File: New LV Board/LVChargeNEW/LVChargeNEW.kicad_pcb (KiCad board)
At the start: 2 copper layers, 54 parts, among them Q1 CSD15380F3T, Q2 CSD15380F3T, Q3 CSD15380F3T, Q4 CSD15380F3T, U1 PQ25856QWRRVRQ1

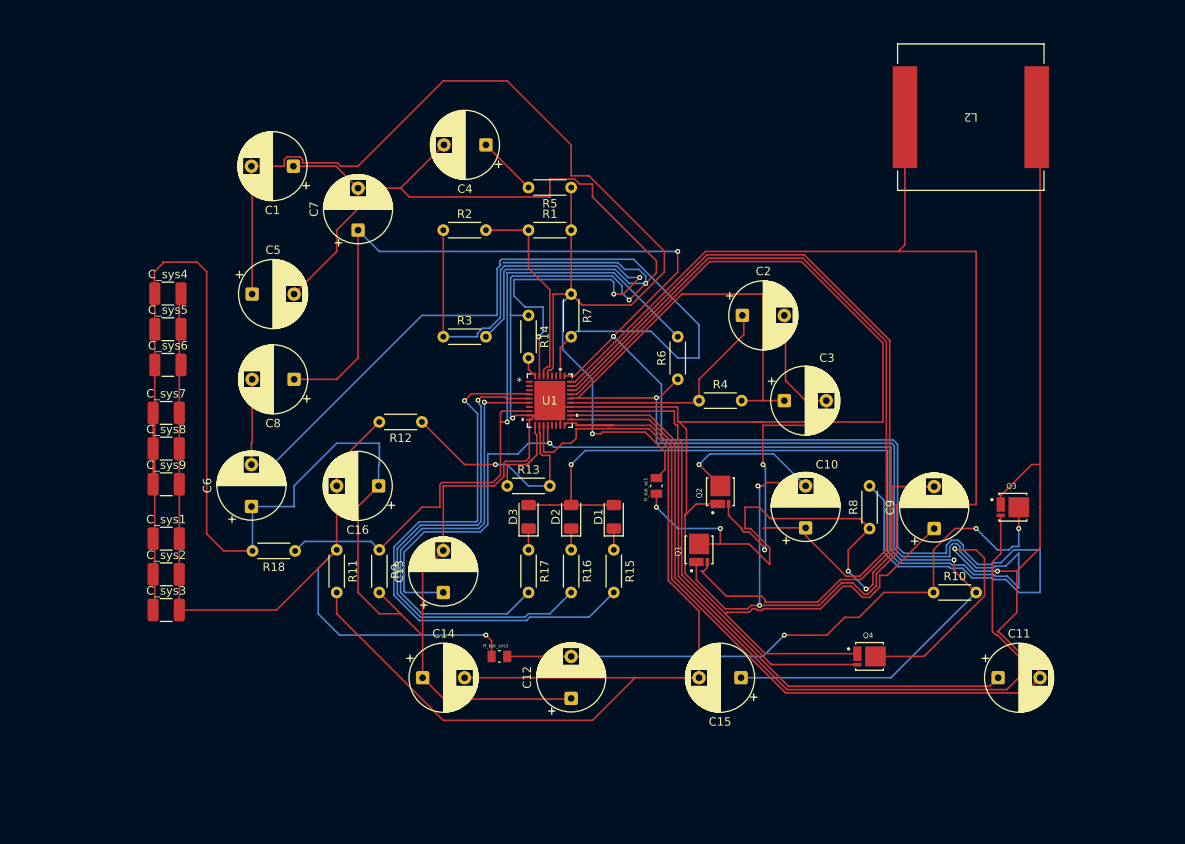
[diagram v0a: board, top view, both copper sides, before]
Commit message: updated LVCharge
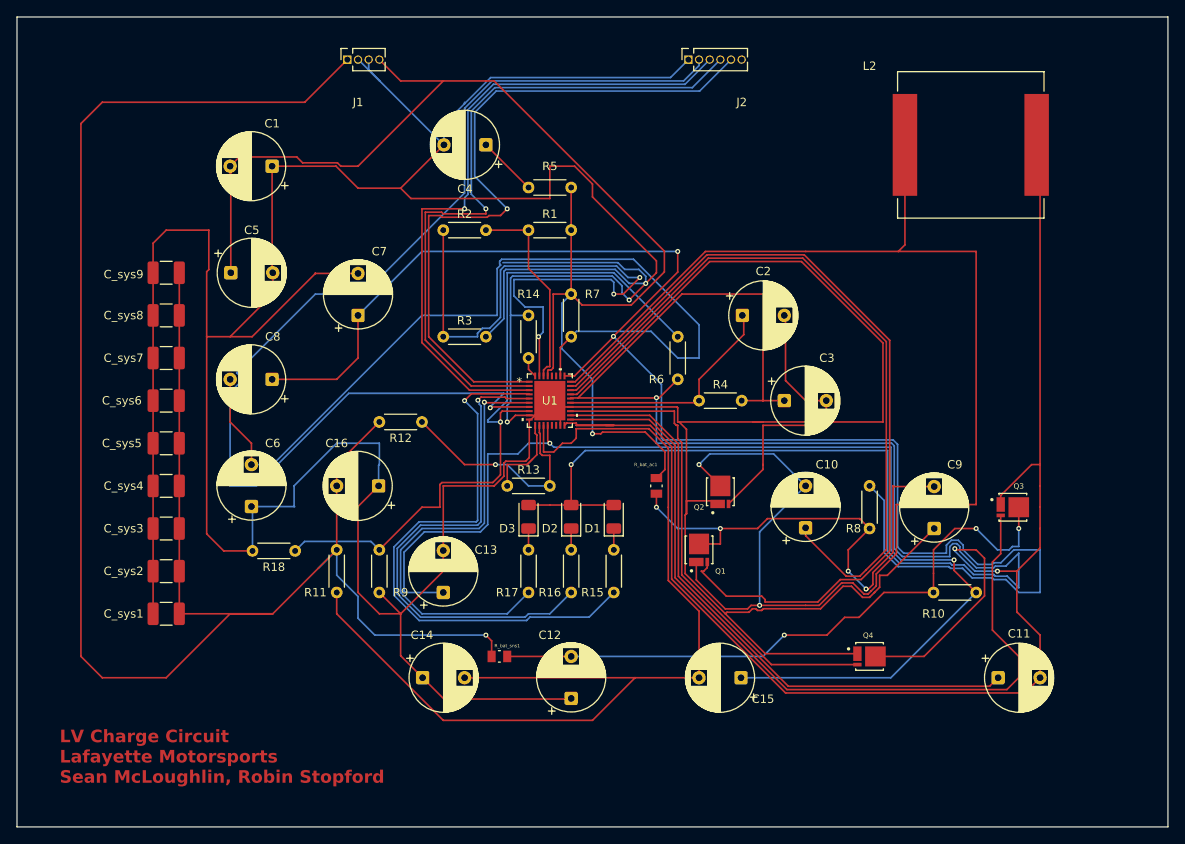
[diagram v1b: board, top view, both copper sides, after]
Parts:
- added J1: Conn_01x04_Socket, Connector_PinSocket_1.27mm:PinSocket_1x04_P1.27mm_Vertical, F.Cu at (80.0, 50.8)
- added J2: Conn_01x05_Socket, Connector_PinSocket_1.27mm:PinSocket_1x06_P1.27mm_Vertical, F.Cu at (120.7, 50.8)
- moved C_sys9 25.2 mm to (58.4, 76.2)
- moved C_sys4 22.9 mm to (58.4, 101.6)
- moved C_sys8 15.9 mm to (58.4, 81.3)
- moved C_sys5 13.6 mm to (58.4, 96.5)
- moved C7 10.2 mm to (81.3, 81.3)
- moved C_sys3 9.71 mm to (58.4, 106.7)
- moved C_sys1 8.95 mm to (58.4, 116.8)
- moved C_sys7 6.55 mm to (58.4, 86.4)
- moved C_sys6 4.26 mm to (58.4, 91.4)
- moved C5 3.59 mm to (66.1, 76.2)
- moved L2 3.30 mm to (154.3, 61.0)
- moved C8 2.62 mm to (71.0, 88.9)
- moved C1 2.54 mm to (71.0, 63.5)
- moved C_sys2 0.38 mm to (58.4, 111.8)
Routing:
- net CE: track 0.00 -> 135.5 mm, vias 0 -> 1
- net Batt+: track 109.3 -> 236.6 mm
- net Batt-: track 515.0 -> 601.6 mm
- net SCL: track 0.00 -> 84.7 mm, vias 0 -> 1
- net SDL: track 0.00 -> 82.4 mm, vias 0 -> 1
- net INT: track 0.00 -> 79.4 mm, vias 0 -> 1
- net Net-(C9-Pad2): track 73.8 -> 61.4 mm
- net Net-(U1-LODRV1): track 94.8 -> 82.9 mm, vias 2 -> 0
- net Buck Input: track 153.4 -> 162.0 mm
- net Net-(U1-ACN): track 194.4 -> 189.0 mm
- net Net-(U1-BTST1): track 92.0 -> 86.9 mm
- net Net-(U1-SW1): track 187.4 -> 184.2 mm, vias 3 -> 2
- net Net-(U1-SW2): track 193.8 -> 191.8 mm
- net Net-(U1-TS): track 83.6 -> 85.3 mm
- net Net-(U1-ACP): track 106.6 -> 107.6 mm
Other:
- board outline added: 137.2 x 96.5 mm
- board text added: "LV Charge Circuit Lafayette Motorsports Sean McLoughlin, Robin Stopford"
